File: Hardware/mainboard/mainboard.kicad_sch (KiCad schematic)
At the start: 9 parts, among them J1 559592430, J2 status bot, J3 status eot, J4 B02B-XASK-1LFSN, U1 S16B-PHDSSLFSN

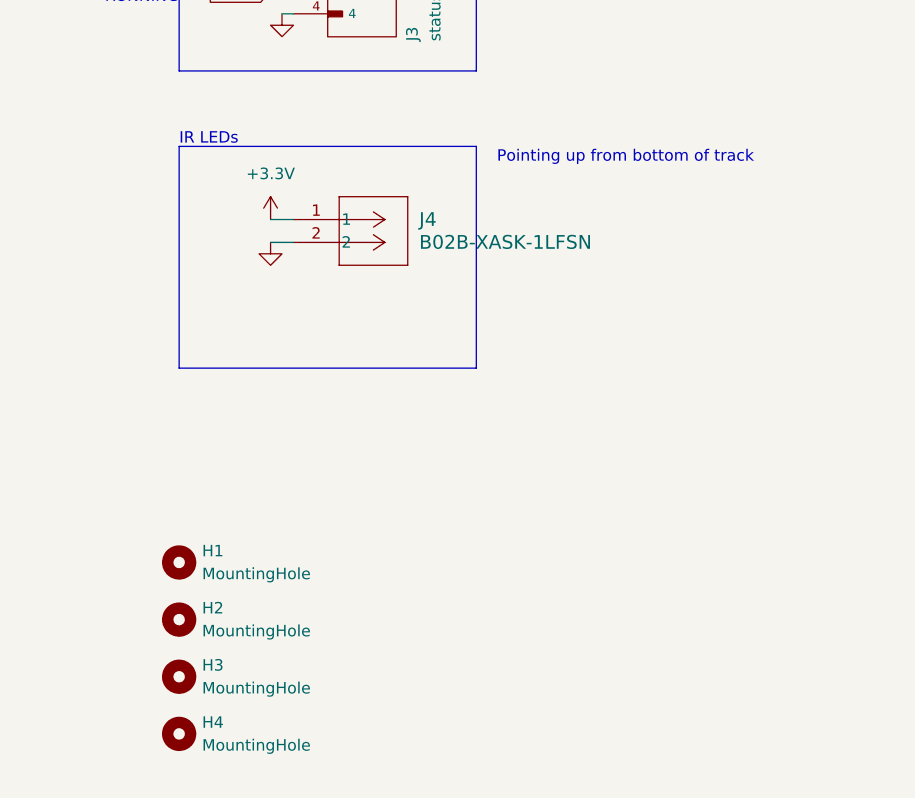
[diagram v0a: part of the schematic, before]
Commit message: generated gbr files
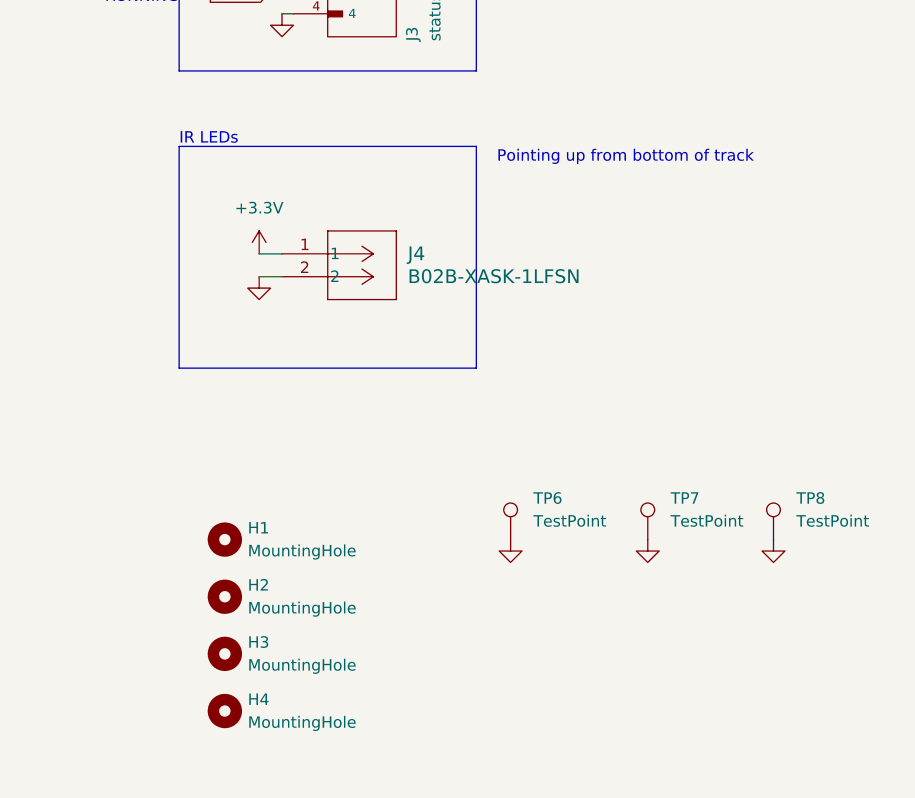
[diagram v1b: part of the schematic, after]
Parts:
- added TP6, TP7, TP8: TestPoint, TestPoint:TestPoint_Keystone_5019_Minature, symbol Connector:TestPoint
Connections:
- net GND: now also TP6.1, TP7.1, TP8.1
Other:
- moved on the sheet: H1, H2, H3, H4, J4
